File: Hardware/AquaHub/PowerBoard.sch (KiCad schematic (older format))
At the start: 20 parts, among them J1 Screw_Terminal_01x02, J2 Screw_Terminal_01x02, J3 Screw_Terminal_01x02, J4 Screw_Terminal_01x02, J5 Screw_Terminal_01x02, J6 Screw_Terminal_01x02, J7 Screw_Terminal_01x02, K1 5A Relay, K2 5A Relay, K3 5A Relay, K4 5A Relay, K5 5A Relay, K6 5A Relay, U2 Current Sense

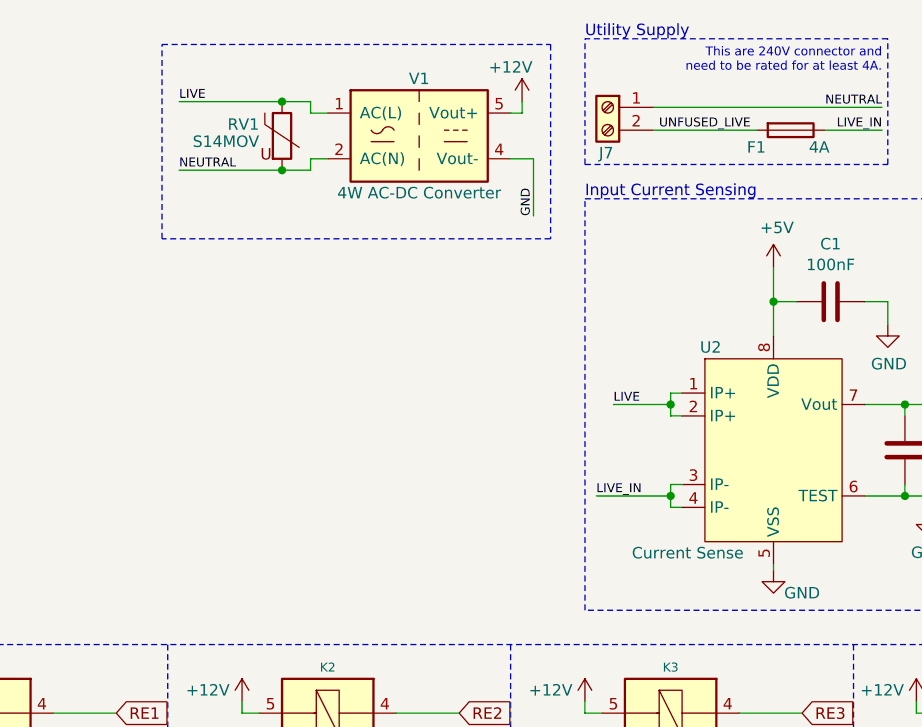
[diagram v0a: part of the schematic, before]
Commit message: Finalising the Rev2 hardware.
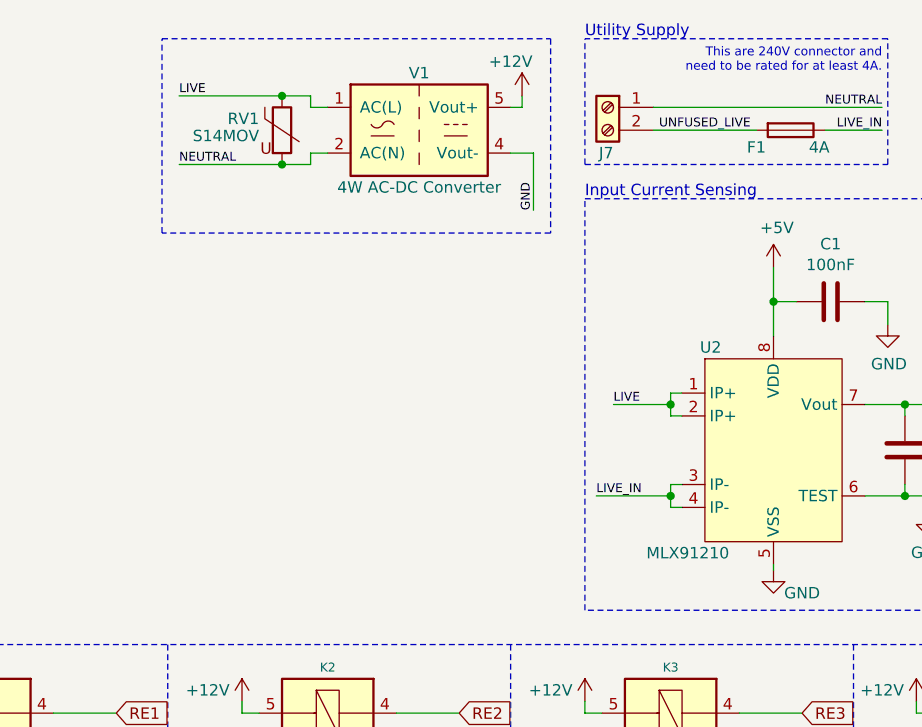
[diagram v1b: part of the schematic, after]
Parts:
- C1: Mouser (none) -> 710-885012206071
- C2, J1, J2, J3, J4, J5, J6, J7, K1, K2, K3, K4, K5, K6, RV1: manf# x -> (none)
- F1: footprint AquaFootprints:Fuse_Clip_5mm -> Fuse:Fuseholder_Glass_5mmx20mm; Mouser (none) -> 534-3512
- R1: Mouser GWCR0603-10KFT5 -> 603-RC0603FR-0710KL
- U2: value Current Sense -> MLX91210; manf# x -> (none)
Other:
- moved on the sheet: RV1, V1
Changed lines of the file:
@@
 F 4 "Mouser" H -900 -450 50  0001 C CNN "Vendor"
 F 5 "FTR-F1AA012V" H 0   0   50  0001 C CNN "Mouser"
-F 6 "x" H 0   0   50  0001 C CNN "manf#"
 	1    3450 5525
 	1    0    0    -1
@@
 F 4 "Mouser" H -900 -450 50  0001 C CNN "Vendor"
 F 5 "FTR-F1AA012V" H 0   0   50  0001 C CNN "Mouser"
-F 6 "x" H 0   0   50  0001 C CNN "manf#"
 	1    4950 5525
 	1    0    0    -1
@@
 F 4 "Mouser" H -900 -450 50  0001 C CNN "Vendor"
 F 5 "FTR-F1AA012V" H 0   0   50  0001 C CNN "Mouser"
-F 6 "x" H 0   0   50  0001 C CNN "manf#"
 	1    6450 5525
 	1    0    0    -1
@@
 F 4 "Mouser" H -900 -450 50  0001 C CNN "Vendor"
 F 5 "FTR-F1AA012V" H 0   0   50  0001 C CNN "Mouser"
-F 6 "x" H 0   0   50  0001 C CNN "manf#"
 	1    7950 5525
 	1    0    0    -1
@@
 F 4 "Mouser" H -900 -450 50  0001 C CNN "Vendor"
 F 5 "FTR-F1AA012V" H 0   0   50  0001 C CNN "Mouser"
-F 6 "x" H 0   0   50  0001 C CNN "manf#"
 	1    9450 5525
 	1    0    0    -1
@@
 F 4 "Mouser" H -900 -450 50  0001 C CNN "Vendor"
 F 5 "FTR-F1AA012V" H 0   0   50  0001 C CNN "Mouser"
-F 6 "x" H 0   0   50  0001 C CNN "manf#"
 	1    1950 5525
 	1    0    0    -1
@@
 F 4 "Mouser" H 325 1175 50  0001 C CNN "Vendor"
 F 5 "1935161" H 0   0   50  0001 C CNN "Mouser"
-F 6 "x" H 0   0   50  0001 C CNN "manf#"
 	1    8200 4575
 	-1   0    0    1
@@
 F 4 "Mouser" H 325 1175 50  0001 C CNN "Vendor"
 F 5 "1935161" H 0   0   50  0001 C CNN "Mouser"
-F 6 "x" H 0   0   50  0001 C CNN "manf#"
 	1    8200 4350
 	-1   0    0    1
@@
 F 4 "Mouser" H 325 1175 50  0001 C CNN "Vendor"
 F 5 "1935161" H 0   0   50  0001 C CNN "Mouser"
-F 6 "x" H 0   0   50  0001 C CNN "manf#"
 	1    8200 4125
 	-1   0    0    1
@@
 F 4 "Mouser" H 325 1175 50  0001 C CNN "Vendor"
 F 5 "1935161" H 0   0   50  0001 C CNN "Mouser"
-F 6 "x" H 0   0   50  0001 C CNN "manf#"
 	1    8200 3900
 	-1   0    0    1
@@
 F 4 "Mouser" H 325 1175 50  0001 C CNN "Vendor"
 F 5 "1935161" H 0   0   50  0001 C CNN "Mouser"
-F 6 "x" H 0   0   50  0001 C CNN "manf#"
 	1    8200 3675
 	-1   0    0    1
@@
 F 4 "Mouser" H 325 1175 50  0001 C CNN "Vendor"
 F 5 "1935161" H 0   0   50  0001 C CNN "Mouser"
-F 6 "x" H 0   0   50  0001 C CNN "manf#"
 	1    8200 3450
 	-1   0    0    1
@@
 F 4 "Mouser" H 1500 -4450 50  0001 C CNN "Vendor"
 F 5 "1935161" H 0   0   50  0001 C CNN "Mouser"
-F 6 "x" H 0   0   50  0001 C CNN "manf#"
 	1    4675 2675
 	-1   0    0    -1
@@
 F 0 "F1" V 5550 2625 50  0000 C CNN
 F 1 "4A" V 5550 2900 50  0000 C CNN
-F 2 "AquaFootprints:Fuse_Clip_5mm" H 5525 2575 50  0001 L CNN
+F 2 "Fuse:Fuseholder_Glass_5mmx20mm" H 5525 2575 50  0001 L CNN
 F 3 "~" H 5475 2775 50  0001 C CNN
 F 4 "Mouser" H 1500 -4450 50  0001 C CNN "Vendor"
+F 5 "534-3512" H 0   0   50  0001 C CNN "Mouser"
 	1    5475 2775
 	0    1    1    0
@@
 AR Path="/5B8F2634/5BD289CE" Ref="U2"  Part="1"
 F 0 "U2" H 5125 4625 50  0000 C CNN
-F 1 "Current Sense" H 5025 3725 50  0000 C CNN
+F 1 "MLX91210" H 5025 3725 50  0000 C CNN
 F 2 "Package_SO:SOIC-8_3.9x4.9mm_P1.27mm" H 5500 3825 50  0001 L CIN
 F 3 "http://www.allegromicro.com/~/media/Files/Datasheets/ACS723-Datasheet.ashx?la=en" H 5400 4175 50  0001 C CNN
 F 4 "Mouser" H -4100 1375 50  0001 C CNN "Vendor"
 F 5 "MLX91210KDC-CAS-102-SP" H 0   0   50  0001 C CNN "Mouser"
-F 6 "x" H 0   0   50  0001 C CNN "manf#"
 	1    5400 4175
 	1    0    0    -1
@@
 F 4 "Mouser" H -4100 1375 50  0001 C CNN "Vendor"
 F 5 "VJ0603A102GXAPW1BC" H 0   0   50  0001 C CNN "Mouser"
-F 6 "x" H 0   0   50  0001 C CNN "manf#"
 	1    5975 4175
 	1    0    0    -1
@@
 F 4 "Mouser" H -4100 1375 50  0001 C CNN "Vendor"
 F 5 "CA07658" H 0   0   50  0001 C CNN "Farnell"
+F 6 "710-885012206071" H 0   0   50  0001 C CNN "Mouser"
 	1    5650 3525
 	0    1    1    0
@@
 F 3 "~" H 6375 4200 50  0001 C CNN
 F 4 "Mouser" H -4100 1375 50  0001 C CNN "Vendor"
-F 5 "GWCR0603-10KFT5" H 0   0   50  0001 C CNN "Mouser"
+F 5 "603-RC0603FR-0710KL" H 0   0   50  0001 C CNN "Mouser"
 	1    6375 4200
 	1    0    0    -1
@@
 L AquaHub-rescue:RAC04-xxGA-Converter_ACDC V?
 U 1 1 5BD6ED98
-P 3850 2800
+P 3850 2775
 AR Path="/5BD6ED98" Ref="V?"  Part="1"
 AR Path="/5B8F2634/5BD6ED98" Ref="V1"  Part="1"
-F 0 "V1" H 3850 3050 50  0000 C CNN
-F 1 "4W AC-DC Converter" H 3850 2550 50  0000 C CNN
-F 2 "Converter_ACDC:Converter_ACDC_RECOM_RAC04-xxSGx_THT" H 3700 2800 50  0001 C CNN
-F 3 "" H 3700 2800 50  0001 C CNN
-F 4 "RAC04-12SGB" H 0   0   50  0001 C CNN "Mouser"
-	1    3850 2800
+F 0 "V1" H 3850 3025 50  0000 C CNN
+F 1 "4W AC-DC Converter" H 3850 2525 50  0000 C CNN
+F 2 "Converter_ACDC:Converter_ACDC_RECOM_RAC04-xxSGx_THT" H 3700 2775 50  0001 C CNN
+F 3 "" H 3700 2775 50  0001 C CNN
+F 4 "RAC04-12SGB" H 0   -25 50  0001 C CNN "Mouser"
+	1    3850 2775
 	1    0    0    -1
 $EndComp
@@
 L AquaHub-rescue:+12V-power #PWR?
 U 1 1 5BD6ED9E
-P 4300 2650
+P 4300 2625
 AR Path="/5BD6ED9E" Ref="#PWR?"  Part="1"
 AR Path="/5B8F2634/5BD6ED9E" Ref="#PWR021"  Part="1"
-F 0 "#PWR021" H 4300 2500 50  0001 C CNN
-F 1 "+12V" H 4250 2800 50  0000 C CNN
-F 2 "" H 4300 2650 50  0001 C CNN
-F 3 "" H 4300 2650 50  0001 C CNN
-	1    4300 2650
-	1    0    0    -1
-$EndComp
-Wire Wire Line
-	4300 2650 4300 2700
+F 0 "#PWR021" H 4300 2475 50  0001 C CNN
+F 1 "+12V" H 4250 2775 50  0000 C CNN
+F 2 "" H 4300 2625 50  0001 C CNN
+F 3 "" H 4300 2625 50  0001 C CNN
+	1    4300 2625
+	1    0    0    -1
+$EndComp
+Wire Wire Line
+	4300 2625 4300 2675
 $Comp
 L AquaHub-rescue:Varistor-Device RV?
 U 1 1 5BD6EDA8
-P 3250 2800
+P 3250 2775
 AR Path="/5BD6EDA8" Ref="RV?"  Part="1"
 AR Path="/5B8F2634/5BD6EDA8" Ref="RV1"  Part="1"
-F 0 "RV1" H 3150 2850 50  0000 R CNN
-F 1 "S14MOV" H 3150 2775 50  0000 R CNN
-F 2 "Varistor:RV_Disc_D15.5mm_W6.1mm_P7.5mm" V 3180 2800 50  0001 C CNN
-F 3 "~" H 3250 2800 50  0001 C CNN
-F 4 "Mouser" H -5150 -1625 50  0001 C CNN "Vendor"
-F 5 "B72214P2251K101" H 0   0   50  0001 C CNN "Mouser"
-F 6 "x" H 0   0   50  0001 C CNN "manf#"
-	1    3250 2800
-	1    0    0    -1
-$EndComp
-Wire Wire Line
-	3375 2700 3375 2650
-Wire Wire Line
-	3375 2650 3250 2650
-Wire Wire Line
-	3375 2900 3375 2950
-Wire Wire Line
-	3375 2950 3250 2950
-Connection ~ 3250 2650
-Connection ~ 3250 2950
-Wire Wire Line
-	3250 2950 2800 2950
-Wire Wire Line
-	3375 2700 3450 2700
-Wire Wire Line
-	3375 2900 3450 2900
-Wire Wire Line
-	4350 2900 4250 2900
-Wire Wire Line
-	4300 2700 4250 2700
-Wire Wire Line
-	4350 2900 4350 3150
-Text Label 4350 3150 1    39   ~ 0
+F 0 "RV1" H 3150 2825 50  0000 R CNN
+F 1 "S14MOV" H 3150 2750 50  0000 R CNN
+F 2 "Varistor:RV_Disc_D15.5mm_W6.1mm_P7.5mm" V 3180 2775 50  0001 C CNN
+F 3 "~" H 3250 2775 50  0001 C CNN
+F 4 "Mouser" H -5150 -1650 50  0001 C CNN "Vendor"
+F 5 "B72214P2251K101" H 0   -25 50  0001 C CNN "Mouser"
+	1    3250 2775
+	1    0    0    -1
+$EndComp
+Wire Wire Line
+	3375 2675 3375 2625
+Wire Wire Line
+	3375 2625 3250 2625
+Wire Wire Line
+	3375 2875 3375 2925
+Wire Wire Line
+	3375 2925 3250 2925
+Connection ~ 3250 2625
+Connection ~ 3250 2925
+Wire Wire Line
+	3250 2925 2800 2925
+Wire Wire Line
+	3375 2675 3450 2675
+Wire Wire Line
+	3375 2875 3450 2875
+Wire Wire Line
+	4350 2875 4250 2875
+Wire Wire Line
+	4300 2675 4250 2675
+Wire Wire Line
+	4350 2875 4350 3125
+Text Label 4350 3125 1    39   ~ 0
 GND
 Wire Wire Line
-	2800 2650 3250 2650
-Text Label 2800 2650 0    39   ~ 0
+	2800 2625 3250 2625
+Text Label 2800 2625 0    39   ~ 0
 LIVE
-Text Label 2800 2950 0    39   ~ 0
+Text Label 2800 2925 0    39   ~ 0
 NEUTRAL
 Wire Notes Line
-	2725 2400 4425 2400
-Wire Notes Line
-	4425 2400 4425 3250
-Wire Notes Line
-	4425 3250 2725 3250
-Wire Notes Line
-	2725 3250 2725 2400
+	2725 2375 4425 2375
+Wire Notes Line
+	4425 2375 4425 3225
+Wire Notes Line
+	4425 3225 2725 3225
+Wire Notes Line
+	2725 3225 2725 2375
 $Comp
 L AquaHub-rescue:PWR_FLAG-power #FLG?
